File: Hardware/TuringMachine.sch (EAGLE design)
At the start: 83 parts, among them IC1 TL072P, IC2 4015, IC3 4015, IC5 4016, IC6 TL072P, IC7 TL072P, T1 2N3904, T2 2N3904, T3 2N3904

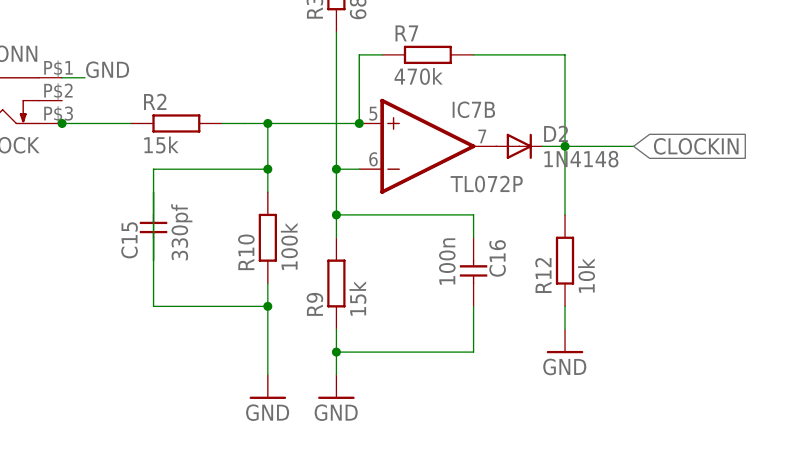
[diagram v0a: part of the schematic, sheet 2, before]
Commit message: routing
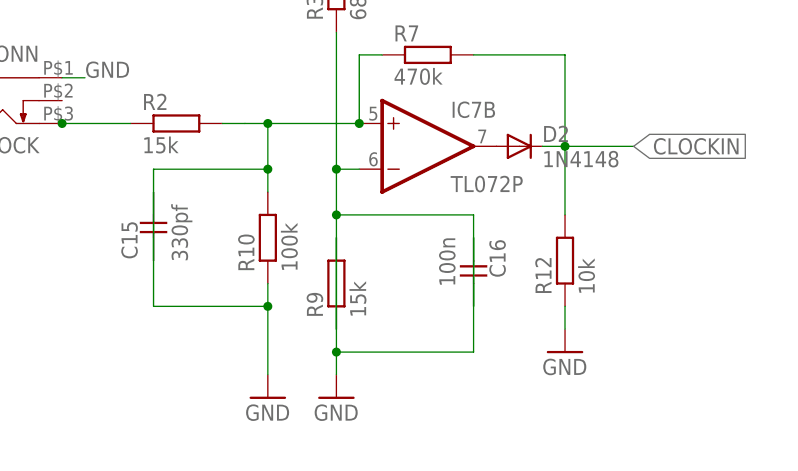
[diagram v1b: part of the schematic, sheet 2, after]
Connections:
- net GND: now also C16.2, R9.2; no longer C16.1, R9.1
- net N$12: now also C16.1, R9.1; no longer C16.2, R9.2
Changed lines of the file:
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@@
 <?xml version="1.0" encoding="utf-8"?>
 <!DOCTYPE eagle SYSTEM "eagle.dtd">
-<eagle version="7.2.0">
+<eagle version="6.6.0">
 <drawing>
 <settings>
@@
 </segment>
 <segment>
-<pinref part="R9" gate="G$1" pin="1"/>
+<pinref part="R9" gate="G$1" pin="2"/>
 <pinref part="GND2" gate="1" pin="GND"/>
 <wire x1="330.2" y1="48.26" x2="330.2" y2="50.8" width="0.1524" layer="91"/>
-<wire x1="330.2" y1="50.8" x2="330.2" y2="53.34" width="0.1524" layer="91"/>
+<wire x1="330.2" y1="50.8" x2="330.2" y2="63.5" width="0.1524" layer="91"/>
 <wire x1="330.2" y1="50.8" x2="345.44" y2="50.8" width="0.1524" layer="91"/>
 <junction x="330.2" y="50.8"/>
-<pinref part="C16" gate="G$1" pin="1"/>
-<wire x1="345.44" y1="50.8" x2="345.44" y2="55.88" width="0.1524" layer="91"/>
+<pinref part="C16" gate="G$1" pin="2"/>
+<wire x1="345.44" y1="50.8" x2="345.44" y2="63.5" width="0.1524" layer="91"/>
 </segment>
 <segment>
@@
 <net name="N$12" class="0">
 <segment>
-<pinref part="R9" gate="G$1" pin="2"/>
+<pinref part="R9" gate="G$1" pin="1"/>
 <pinref part="R3" gate="G$1" pin="1"/>
 <wire x1="330.2" y1="86.36" x2="330.2" y2="71.12" width="0.1524" layer="91"/>
 <pinref part="IC7" gate="B" pin="-IN"/>
 <wire x1="330.2" y1="71.12" x2="330.2" y2="66.04" width="0.1524" layer="91"/>
-<wire x1="330.2" y1="66.04" x2="330.2" y2="63.5" width="0.1524" layer="91"/>
+<wire x1="330.2" y1="66.04" x2="330.2" y2="53.34" width="0.1524" layer="91"/>
 <wire x1="332.74" y1="71.12" x2="330.2" y2="71.12" width="0.1524" layer="91"/>
 <junction x="330.2" y="71.12"/>
 <wire x1="330.2" y1="66.04" x2="345.44" y2="66.04" width="0.1524" layer="91"/>
 <junction x="330.2" y="66.04"/>
-<pinref part="C16" gate="G$1" pin="2"/>
-<wire x1="345.44" y1="66.04" x2="345.44" y2="63.5" width="0.1524" layer="91"/>
-</segment>
-</net>
+<pinref part="C16" gate="G$1" pin="1"/>
+<wire x1="345.44" y1="66.04" x2="345.44" y2="55.88" width="0.1524" layer="91"/>
+</segment>
+</net>
